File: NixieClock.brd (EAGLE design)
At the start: 138 x 60 mm, 65 parts, among them IC1 SN75468D, IC11 TPS73633DBVT, IC12 MCP111T-300E/TT, IC13 MAX1771ESA+, IC2 SN75468D, IC3 SN75468D, IC4 SN75468D, IC5 SN74HC595PW, IC6 SN74HC595PW, IC7 SN74HC595PW, IC8 SN74HC595PW, J1 PCB Terminal, J2 PCB Terminal, J3 501568-0607, M1 JTAG-10PIN-ARM-CONN, Q1 NIXIE-IN-8-2, Q2 NIXIE-IN-8-2, Q3 NIXIE-IN-8-2, Q4 NIXIE-IN-8-2, Q5 BF820, Q6 BF821, Q7 FQD16N25CTM, Q8 BF820, U1 TM4C1231H6PMI7, Y1 16 MHz, Y2 32.768 kHz

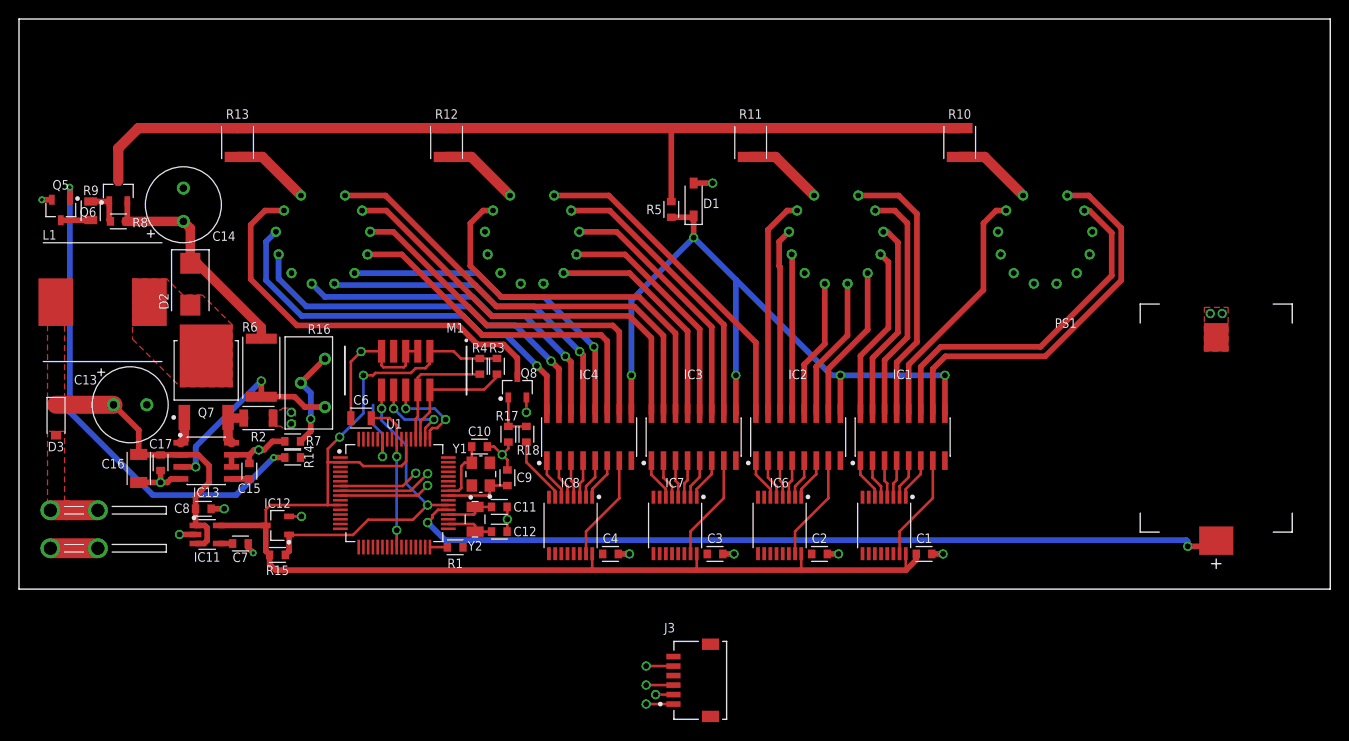
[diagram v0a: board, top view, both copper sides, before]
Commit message: Update
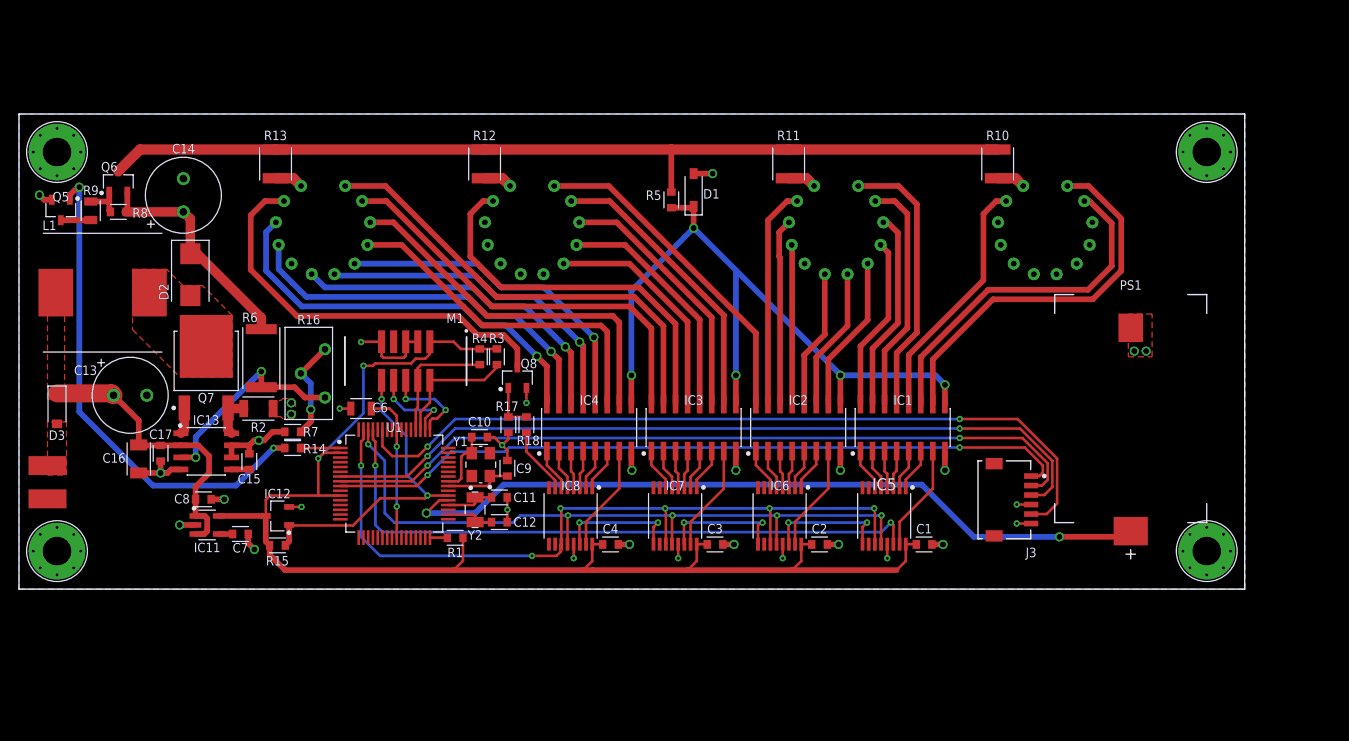
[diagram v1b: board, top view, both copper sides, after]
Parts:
- added MT1, MT2, MT3, MT4: MOUNTING_HOLE_3MM, Misc:MOUNTING_HOLE_3MM
- J1, J2: device Connectors:PCB_TERMINAL_2.8X0.81_RGIHT_ANGLE -> Connectors:PCB_TERMINAL_PAD
- moved J3 37.2 mm to (103.7, 9.40), turned to 180 degrees
- moved PS1 9.06 mm to (117.0, 19.0)
- moved J2 5.91 mm to (3.00, 9.50)
- moved J1 5.47 mm to (3.00, 13.0)
- moved R10 4.59 mm to (103.0, 44.8)
- moved R11 4.59 mm to (81.0, 44.8)
- moved R12 4.59 mm to (49.0, 44.8)
- moved R13 4.59 mm to (27.0, 44.8)
- moved D3 1.20 mm to (4.00, 19.0)
- moved C1 1.00 mm to (95.2, 4.70)
- moved C10 1.00 mm to (48.5, 16.0)
- moved C11 1.00 mm to (50.5, 9.65)
- moved C12 1.00 mm to (50.5, 7.05)
- moved C13 1.00 mm to (11.7, 20.4)
- moved C14 1.00 mm to (17.3, 41.5)
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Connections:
- net N$39 renamed SW_3
- net N$40 renamed SW_2
- net N$41 renamed SW_1
- net N$43 renamed LIGHT_SEN
- net GND: now also MT1.0, MT1.1, MT1.2, MT1.3, MT1.4, MT1.5, MT1.6, MT1.7, MT1.8, MT2.0, MT2.1, MT2.2, MT2.3, MT2.4, MT2.5, MT2.6, MT2.7, MT2.8, MT3.0, MT3.1, MT3.2, MT3.3, MT3.4, MT3.5, MT3.6, MT3.7, MT3.8, MT4.0, MT4.1, MT4.2, MT4.3, MT4.4, MT4.5, MT4.6, MT4.7, MT4.8; no longer J2.2
- net VSUPP: no longer J1.2
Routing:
- net SR_SRCLK: track 0.00 -> 82.4 mm, vias 0 -> 6
- net SR_RCLK: track 0.00 -> 74.7 mm, vias 0 -> 5
- net LIGHT_SEN: track 10.5 -> 84.4 mm
- net SW_1: track 11.4 -> 83.8 mm
- net SW_2: track 11.8 -> 81.1 mm
- net SR_SER: track 0.00 -> 67.5 mm, vias 0 -> 2
- net SW_3: track 12.5 -> 78.5 mm
- net N$16: track 0.00 -> 13.1 mm, vias 0 -> 2
- net N$8: track 0.00 -> 13.0 mm, vias 0 -> 2
- net N$24: track 0.00 -> 13.0 mm, vias 0 -> 2
- net GND: track 58.7 -> 65.6 mm, vias 20 -> 31
- net VBAT: track 87.5 -> 80.8 mm
- net N$76: track 8.36 -> 3.01 mm
- net N$75: track 8.36 -> 3.01 mm
- net N$74: track 8.36 -> 3.01 mm
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- added copper zone on layer 16, net GND
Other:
- board size 138 x 60 mm -> 129 x 50 mm

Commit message: Update
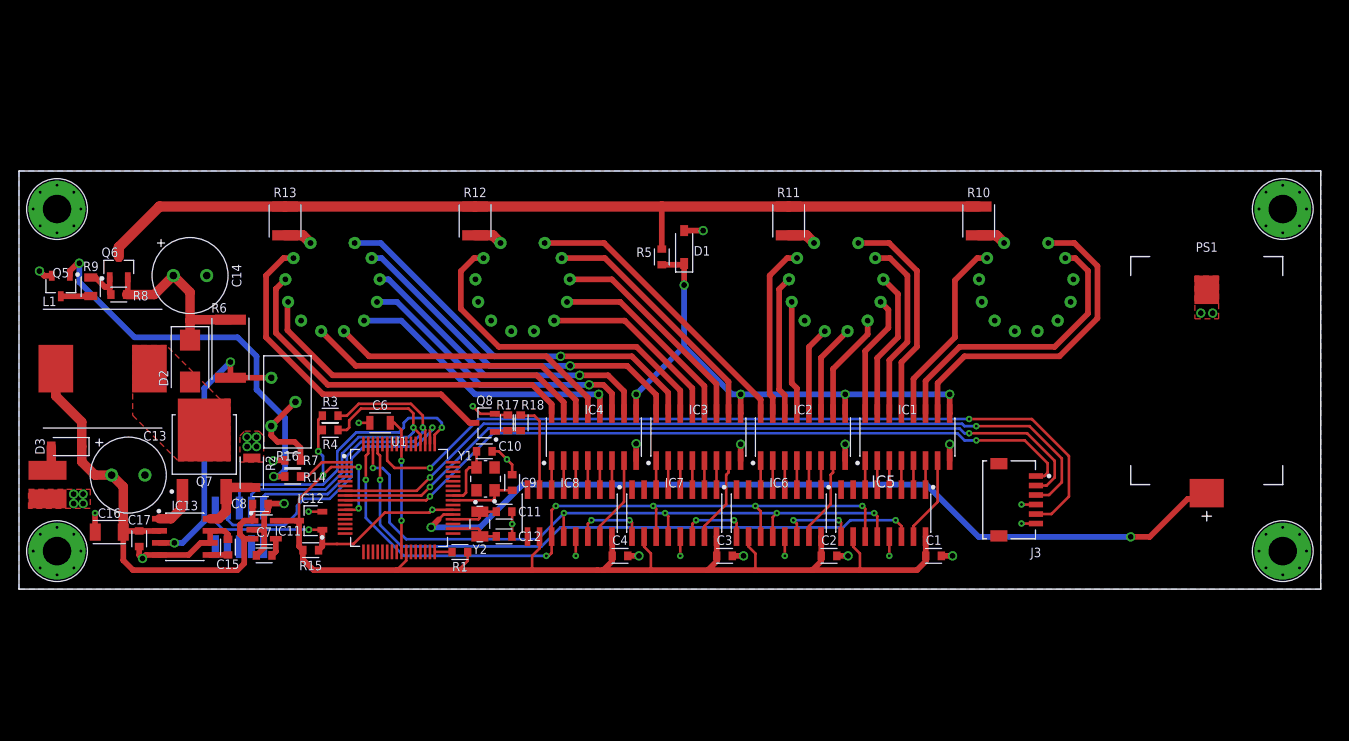
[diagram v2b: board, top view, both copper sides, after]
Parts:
- IC5, IC6, IC7, IC8: value SN74HC595PW -> SN74HC595DR; device ICs:SOP65P640X120-16N -> ICs:SOIC127P600X175-16N
- M1: value JTAG-10PIN-ARM-CONN -> JTAG-ARM-10PIN-PLACEHOLDER; device Connectors:20021521-00010T1LF -> Connectors:JTAG-ARM-10PIN-PLACEHOLDER
- moved M1 24.7 mm to (23.2, 6.50), flipped to the bottom, turned to 0 degrees
- moved R3 18.6 mm to (32.8, 18.2), turned to 180 degrees
- moved R4 17.5 mm to (32.8, 16.8), turned to 180 degrees
- moved MT2 10.0 mm to (133.0, 40.0)
- moved C15 9.28 mm to (22.0, 4.42)
- moved C17 9.28 mm to (12.7, 5.30)
- moved IC13 9.28 mm to (17.4, 5.50)
- moved D2 9.09 mm to (18.0, 24.0)
- moved Q6 9.00 mm to (10.5, 33.9)
- moved PS1 8.94 mm to (125.0, 23.0)
- moved Q7 8.80 mm to (19.5, 14.5)
- moved R8 8.70 mm to (10.5, 31.0)
- moved C14 8.48 mm to (18.0, 33.0), turned to 0 degrees
- moved C13 8.40 mm to (11.5, 12.0)
- moved C16 8.30 mm to (9.50, 6.00), turned to 180 degrees
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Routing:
- net JTAG_TCK: track 13.3 -> 35.9 mm, vias 0 -> 1
- net JTAG_TMS: track 13.5 -> 35.5 mm, vias 0 -> 1
- net DTA_COM: track 78.4 -> 56.5 mm
- net JTAG_TDI: track 9.11 -> 30.8 mm, vias 2 -> 1
- net JTAG_TDO: track 9.69 -> 30.4 mm, vias 2 -> 1
- net 12V: track 31.3 -> 49.8 mm
- net N$80: track 52.0 -> 41.6 mm
- net 3V3: track 140.8 -> 130.5 mm, vias 2 -> 4
- net VBAT: track 80.8 -> 90.6 mm
- net N$68: track 43.3 -> 35.8 mm
- net N$81: track 22.3 -> 29.5 mm
- net N$9: track 41.0 -> 34.5 mm
- net N$10: track 37.4 -> 30.9 mm
- net N$61: track 39.2 -> 32.9 mm, vias 0 -> 1
- net N$60: track 44.0 -> 37.9 mm, vias 0 -> 1
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- removed copper zone on layer 1, net 12V
- removed copper zone on layer 1, net VSUPP
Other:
- board size 129 x 50 mm -> 137 x 44 mm
